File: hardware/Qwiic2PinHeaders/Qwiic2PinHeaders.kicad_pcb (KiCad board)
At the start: 2 copper layers, 10 x 25 mm, 4 parts, among them J1 Conn_01x04_Pin, J2 Qwiic, J3 Qwiic

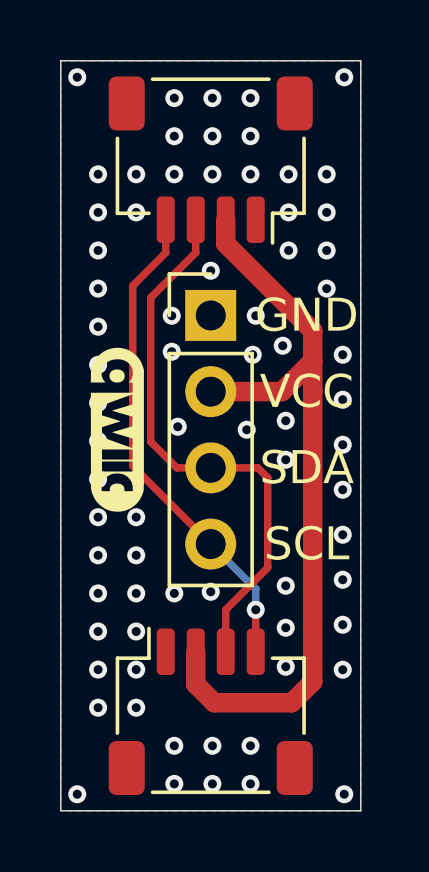
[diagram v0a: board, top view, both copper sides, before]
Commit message: hardware: add misc project files
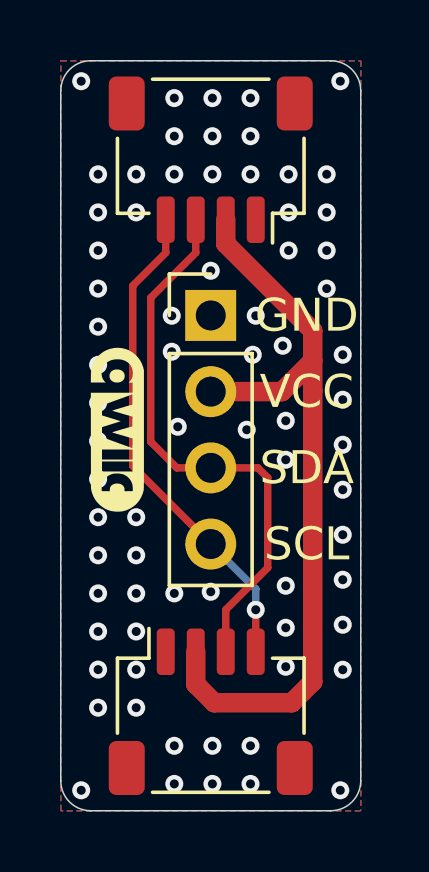
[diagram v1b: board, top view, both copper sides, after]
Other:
- outline, holes or cut-outs redrawn
